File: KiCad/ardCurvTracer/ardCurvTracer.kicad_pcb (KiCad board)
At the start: 2 copper layers, 116.2 x 88.9 mm, 60 parts, among them J1 4-pin_Serial_Connection_header, Q1 BC639, Q2 BC639, Q3 BC639, SW1 On/Off, U1 MCP4802, U2 Test socket, U3 LM358, U5 HT7550, U6 HT7533

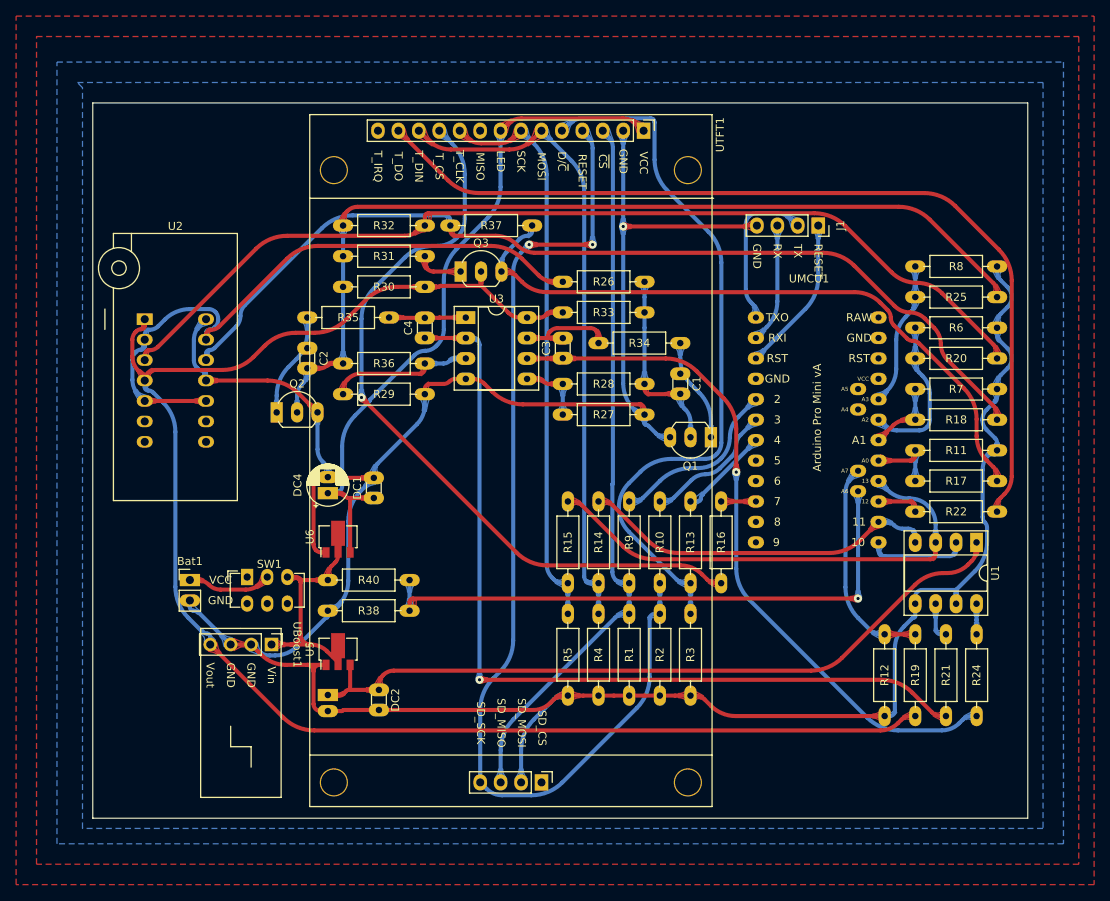
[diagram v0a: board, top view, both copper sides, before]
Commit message: kicad
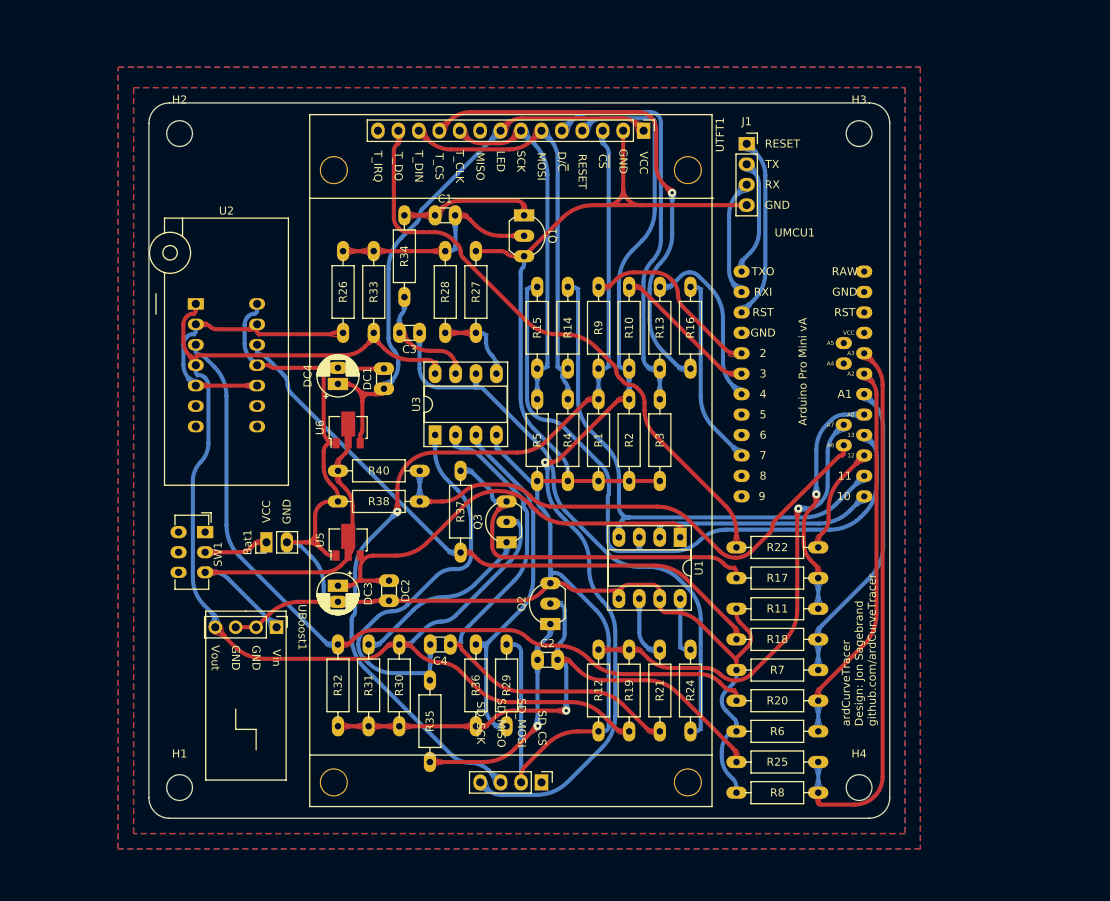
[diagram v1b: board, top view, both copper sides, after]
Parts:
- added H1: MountingHole, MountingHole:MountingHole_3.2mm_M3, F.Cu at (111.8, 132.7)
- added H2: MountingHole, MountingHole:MountingHole_3.2mm_M3, F.Cu at (111.8, 51.4)
- added H3: MountingHole, MountingHole:MountingHole_3.2mm_M3, F.Cu at (196.2, 51.4)
- added H4: MountingHole, MountingHole:MountingHole_3.2mm_M3, F.Cu at (196.2, 132.7)
- DC3: moved to F.Cu
- moved R8 66.5 mm to (191.1, 133.3), turned to 180 degrees
- moved R25 66.2 mm to (181.0, 129.5), turned to 0 degrees
- moved R31 58.5 mm to (135.3, 125.1), turned to 90 degrees
- moved R20 53.5 mm to (181.0, 121.9), turned to 0 degrees
- moved R32 53.2 mm to (131.4, 114.9), turned to -90 degrees
- moved R6 51.6 mm to (191.1, 125.7), turned to 180 degrees
- moved C2 48.2 mm to (156.2, 116.8), turned to 0 degrees
- moved R29 46.0 mm to (152.4, 125.1), turned to 90 degrees
- moved R35 45.4 mm to (142.9, 119.4), turned to -90 degrees
- moved R30 44.6 mm to (139.1, 114.9), turned to -90 degrees
- moved Q2 43.0 mm to (157.8, 112.4), turned to 90 degrees
- moved R18 42.4 mm to (181.0, 114.3), turned to 0 degrees
- moved C4 38.2 mm to (145.4, 114.9), turned to 180 degrees
- moved R26 37.7 mm to (132.1, 66.0), turned to -90 degrees
- moved R7 37.0 mm to (191.1, 118.1), turned to 180 degrees
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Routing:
- net Net-(R25-Pad2): track 18.0 -> 68.5 mm
- net Net-(QNPN1-Pad1): track 82.2 -> 36.8 mm
- net InOpA: track 108.4 -> 64.4 mm, vias 1 -> 0
- net Net-(QNPN1-Pad2): track 119.1 -> 76.0 mm
- net OutOpA: track 115.5 -> 73.5 mm, vias 0 -> 1
- net Net-(C4-Pad2): track 9.55 -> 51.3 mm
- net Net-(R13-Pad2): track 89.1 -> 49.9 mm
- net Net-(R22-Pad2): track 113.7 -> 74.7 mm
- net +5V: track 92.4 -> 54.3 mm
- net Net-(Q3-Pad3): track 83.6 -> 46.2 mm
- net +12V: track 196.6 -> 159.5 mm
- net Net-(R16-Pad2): track 94.8 -> 62.5 mm
- net Net-(R12-Pad1): track 27.1 -> 56.5 mm, vias 0 -> 1
- net Net-(R18-Pad2): track 9.32 -> 38.1 mm
- net Net-(R20-Pad2): track 19.5 -> 47.6 mm
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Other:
- board size 116.2 x 88.9 mm -> 92.1 x 88.9 mm
- board text added: "PNP: 1 -> Collector <- 4 2 -> Base <- 5 3 -> Emitter <- 3 NPN: 12 -> Collector <- 12 10 -> Base <- 13 11 -> Emitter <- 14"
- board text added: "ardCurveTracer Design: Jon Sagebrand github.com/ardCurveTracer"
